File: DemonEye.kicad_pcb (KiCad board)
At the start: 2 copper layers, 16.4 x 35.2 mm, 59 parts, among them CN1 PicoBlade 1x07 P1.25mm, Q1 CSD25501F3, Q2 CSD25501F3, Q3 CSD25501F3, Q4 CSD25501F3, Q5 CSD25501F3, U1 WS2814B

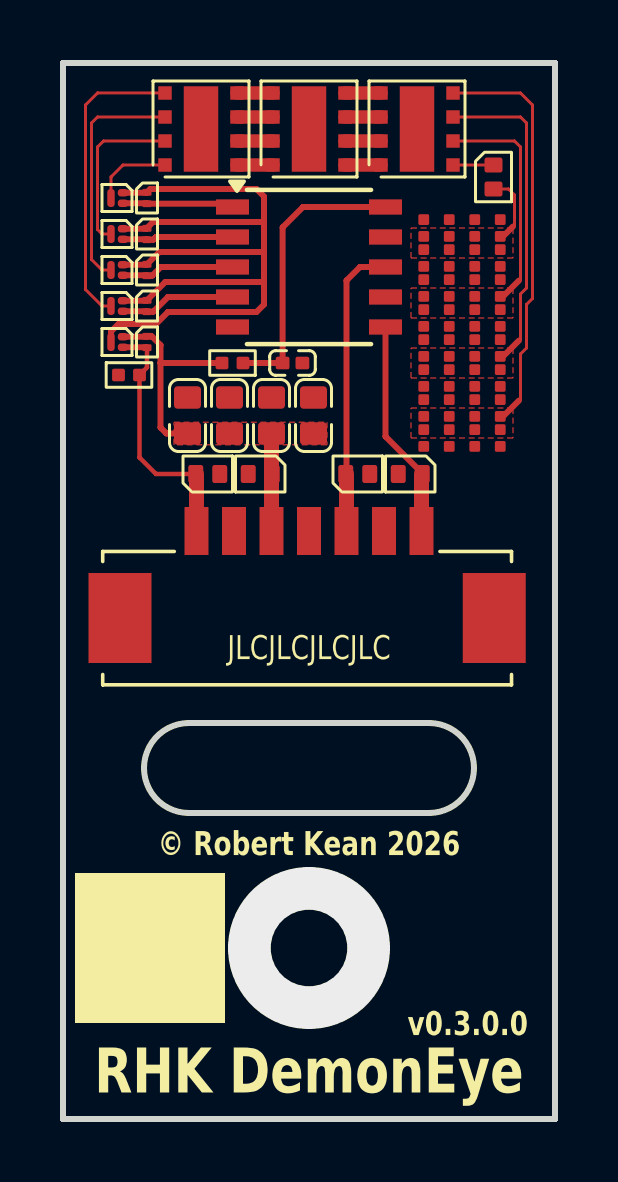
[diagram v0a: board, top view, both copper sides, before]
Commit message: Update .gitignore, DemonEye.kicad_pcb, DemonEye.kicad_prl, and 3 more files
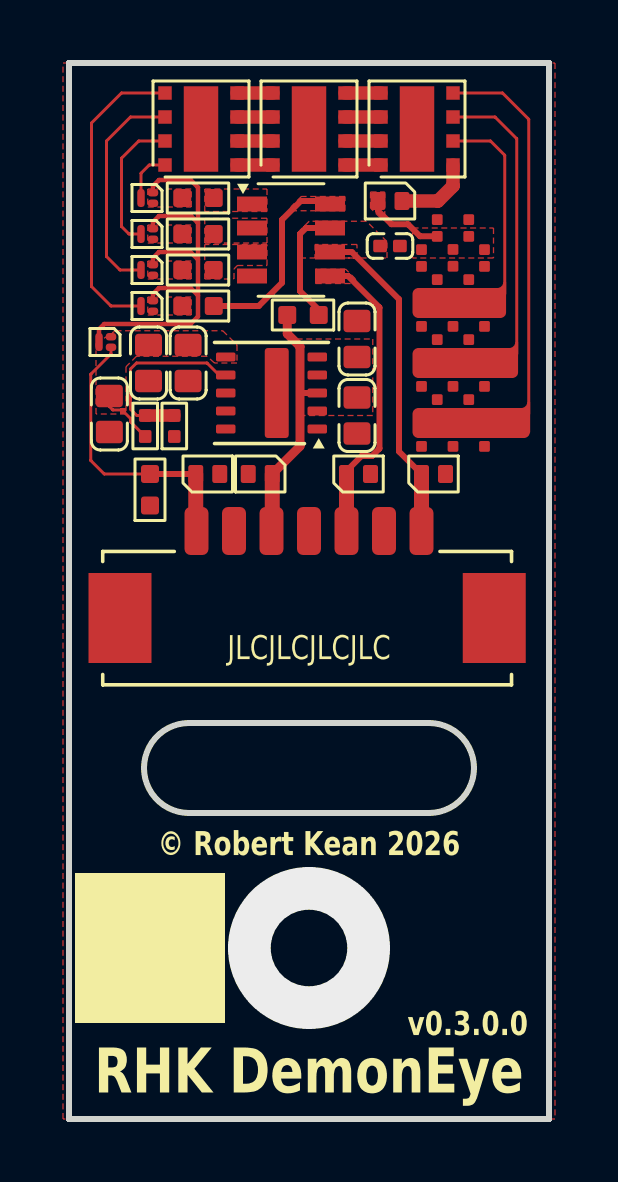
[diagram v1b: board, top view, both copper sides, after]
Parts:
- removed D1, D2, D3, D4, D5: 13V, My Package_Leadless:DFN0603-2
- removed the R10 at (114.0, 65.9)
- removed the R11 at (111.4, 66.9)
- removed the R15 at (111.4, 67.9)
- removed the R18 at (114.0, 67.9)
- removed the R19 at (111.4, 68.9)
- removed the R23 at (111.4, 69.9)
- removed the R26 at (114.0, 69.9)
- removed R31, R34: 680R, My Resistors:R_0201_Dense
- removed the R7 at (111.4, 65.9)
- added C6: 22uF, My Capacitors:C_0603_Dense, F.Cu at (100.9, 71.1)
- added R28: 25k5, My Resistors:R_0201_Nominal, F.Cu at (103.1, 71.5)
- added R4: 1k0, My Resistors:R_0402_Nominal, F.Cu at (103.9, 65.1)
- added R5: 1k0, My Resistors:R_0402_Nominal, F.Cu at (103.9, 66.3)
- added R6: 1k0, My Resistors:R_0402_Nominal, F.Cu at (103.9, 67.5)
- added U2: LMZM23601, My Package_Leadless:Texas_SIL0010A_MicroSiP-10-1EP_3.8x3mm_P0.6mm_EP0.7x2.9mm, F.Cu at (106.3, 70.4)
- R1, R2: value 2k7 -> 1k0; footprint My Resistors:R_0201_Nominal -> My Resistors:R_0402_Nominal
- R10: renamed from R8; value 680R -> 100R
- R11: renamed from R9; value 680R -> 100R
- R12, R13, R14, R16: value 680R -> 100R
- R15: renamed from R17; value 680R -> 100R
- R17: renamed from R20; value 680R -> 100R
- R18: renamed from R21; value 680R -> 100R
- R19: renamed from R22; value 680R -> 100R
- R20: renamed from R24; value 680R -> 100R
- R21: renamed from R25; value 680R -> 100R
- R22: renamed from R28; value 680R -> 100R
- R23: renamed from R29; value 680R -> 100R
- R24: renamed from R30; value 680R -> 100R
- R25: renamed from R32; value 680R -> 100R
- R26: renamed from R33; value 680R -> 100R
- R27: value 680R -> 249k; footprint My Resistors:R_0201_Dense -> My Resistors:R_0201_Nominal
- R3: value 680R -> 1k0; footprint My Resistors:R_0201_Dense -> My Resistors:R_0402_Nominal
- R7: renamed from R4; value 680R -> 100R
- R8: renamed from R5; value 680R -> 100R
- R9: renamed from R6; value 680R -> 100R
- U1: value WS2814B -> WS2814F; footprint Package_SO:SSOP-10_3.9x4.9mm_P1.00mm -> My Package_SO:FSOP-8_3.25x1.65mm_P0.8mm
- moved R27 9.30 mm to (102.1, 71.5), turned to -90 degrees
- moved R3 7.59 mm to (103.9, 63.9), turned to 180 degrees
- moved C3 6.20 mm to (109.2, 68.6)
- moved C1 5.08 mm to (110.3, 65.5)
- moved C5 4.53 mm to (103.6, 69.4), turned to -90 degrees
- moved C4 4.46 mm to (102.2, 69.4), turned to -90 degrees
- moved C2 4.25 mm to (109.2, 71.2), turned to -90 degrees
- moved R1 3.89 mm to (102.3, 73.6), turned to 90 degrees
- moved D10 3.54 mm to (110.3, 64.0), turned to 180 degrees
- moved R2 2.84 mm to (107.4, 67.8)
- moved R14 2.81 mm to (111.3, 67.9), turned to -90 degrees
- moved R19 2.81 mm to (111.3, 69.9), turned to -90 degrees
- moved R24 2.81 mm to (111.3, 71.9), turned to -90 degrees
- moved R9 2.81 mm to (111.3, 65.9), turned to -90 degrees
- moved D7 2.53 mm to (111.8, 73.1)
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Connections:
- net /+12V_{SW} renamed /+V_{OUT_{SW}}
- C4 pad 1: +12V -> V_{OUT}
- C5 pad 1: +12V -> V_{OUT}
- CN1 pad 5: /D_{IN} -> /D_{OUT}
- CN1 pad 7: /D_{OUT} -> /D_{IN}
- Q1 pad 2: +12V -> V_{OUT}
- Q2 pad 1: /OUTR -> /RedG
- Q3 pad 1: /OUTG -> /GreenG
- Q4 pad 1: /OUTB -> /BlueG
- Q5 pad 1: /OUTW -> /WhiteG
- R27 pad 1: /White3 -> /FB
- R27 pad 2: GND -> V_{OUT}
- R3 pad 1: /Red4 -> /OUTR
- R3 pad 2: GND -> /RedG
- U1 pad 4: /OUTW -> GND
- U1 pad 5: GND -> /D_{OUT}
- U1 pad 6: /D_{OUT} -> /D_{IN}
- U1 pad 7: GND -> /V_{DD}
- U1 pad 8: /D_{IN} -> /OUTW
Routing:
- net /+V_{OUT_{SW}}: track 28.9 -> 15.8 mm
- net /FB: track 0.00 -> 6.31 mm
- net /V_{DD}: track 9.55 -> 4.04 mm
- net /OUTB: track 3.78 -> 0.00 mm
- net /OUTR: track 3.70 -> 0.00 mm
- net /OUTG: track 3.69 -> 0.00 mm
- net /D_{OUT}: track 7.30 -> 10.2 mm
- net /OUTW: track 3.86 -> 6.60 mm
- net V_{OUT}: track 0.00 -> 2.18 mm
- net +12V: track 10.4 -> 8.34 mm
- net /Red3: track 1.35 -> 2.61 mm
- net /D_{IN}: track 9.84 -> 11.0 mm
- net /Blue3: track 10.7 -> 9.60 mm
- net /Green3: track 7.62 -> 6.55 mm
- net /SRH: track 8.60 -> 9.65 mm
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- added copper zone on F.Cu, net /BlueG
- added copper zone on F.Cu, net /D_{IN}
- added copper zone on F.Cu, net /D_{OUT}
- added copper zone on F.Cu, net /GreenG
- added copper zone on F.Cu, net /OUTB
- added copper zone on F.Cu, net /OUTG
- added copper zone on F.Cu, net /OUTR
- added copper zone on F.Cu, net /OUTW
- added copper zone on F.Cu, net /RedG
- added copper zone on F.Cu, net /V_{DD}
- added copper zone on F.Cu, net /WhiteG
- added copper zone on F.Cu, net V_{OUT}
- removed copper zone on F.Cu, net /Blue3
- removed copper zone on F.Cu, net /Green3
- removed copper zone on F.Cu, net /White3
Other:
- board size 16.4 x 35.2 mm -> 16 x 35.2 mm
